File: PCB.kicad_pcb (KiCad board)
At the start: 2 copper layers, 100 x 80 mm, 31 parts, among them J1 Conn_01x04_Pin, SW1 SW_Push, SW2 SW_Push, SW3 SW_Push, SW4 SW_Push, SW5 SW_Push, SW6 SW_Push, SW7 RotaryEncoder_Switch, U1 MOUDLE-SEEEDUINO-XIAO

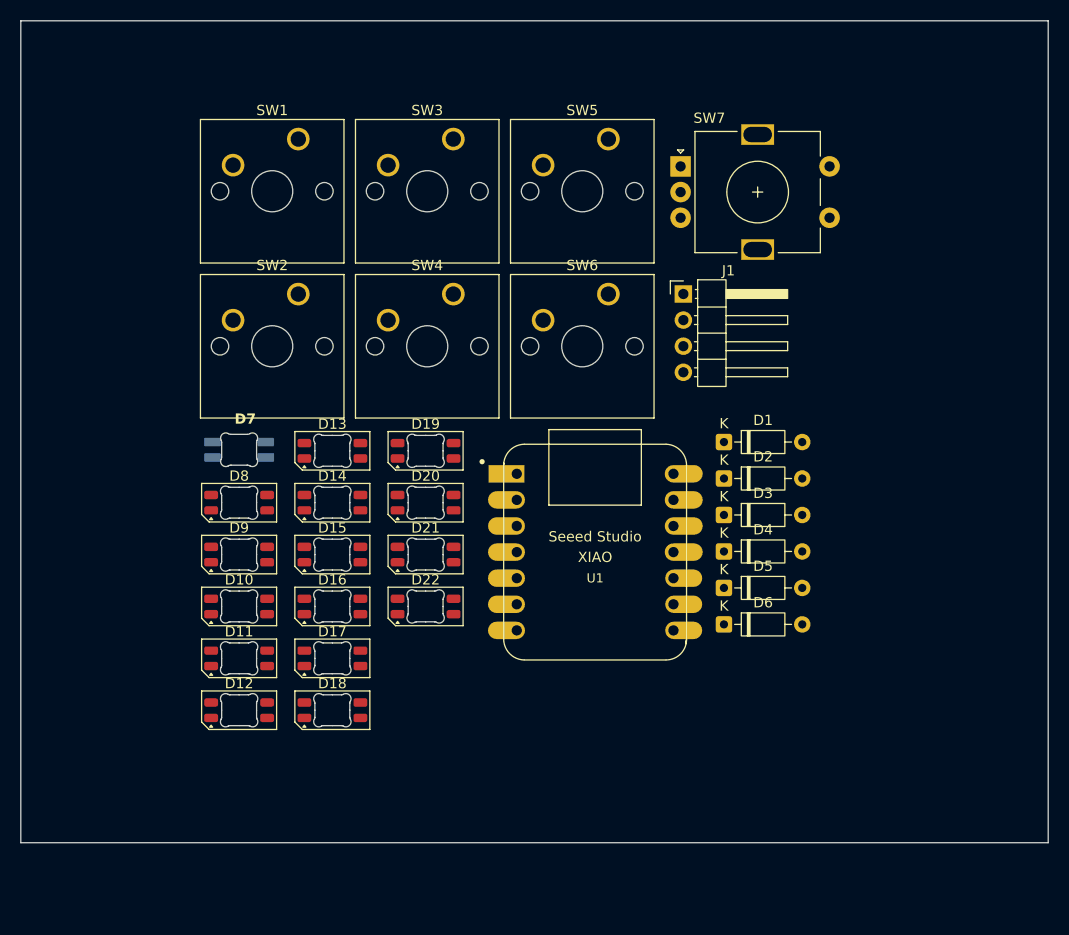
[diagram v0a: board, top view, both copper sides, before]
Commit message: PCB done
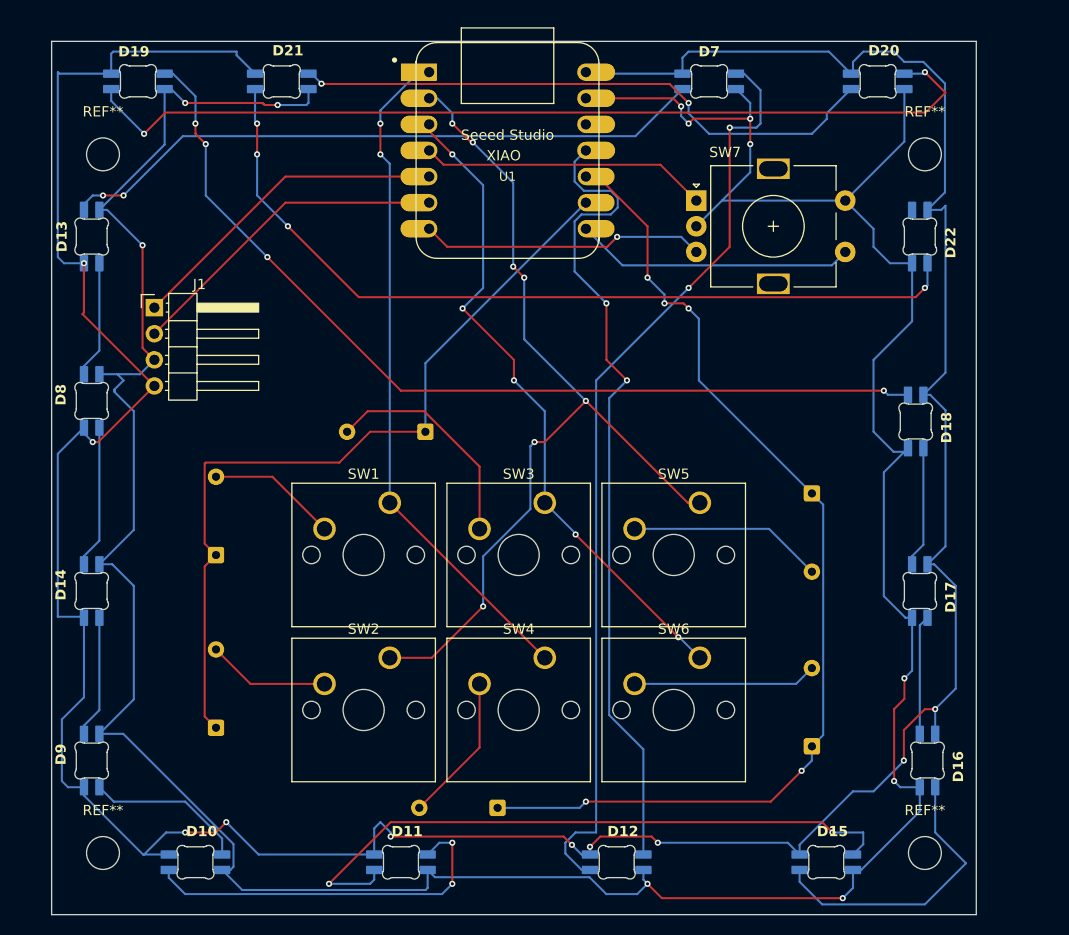
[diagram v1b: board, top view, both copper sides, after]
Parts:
- added REF**: MountingHole_3.2mm_M3, MountingHole:MountingHole_3.2mm_M3, F.Cu at (193.0, 42.0)
- added REF**: MountingHole_3.2mm_M3, MountingHole:MountingHole_3.2mm_M3, F.Cu at (113.0, 110.0)
- added REF**: MountingHole_3.2mm_M3, MountingHole:MountingHole_3.2mm_M3, F.Cu at (193.0, 110.0)
- added REF**: MountingHole_3.2mm_M3, MountingHole:MountingHole_3.2mm_M3, F.Cu at (113.0, 42.0)
- D1, D2, D3, D4, D5, D6: moved to B.Cu
- D10, D11, D12, D13, D14, D15, D16, D17, D18, D19, D20, D21, D22, D8, D9: footprint LED_SMD:LED_SK6812MINI-E_3.2x2.8mm_P1.5mm_ReverseMount -> footprints:SK6812MINI-E_fixed
- moved D18 63.3 mm to (192.0, 68.0), turned to -90 degrees
- moved D20 60.1 mm to (188.4, 35.0)
- moved D22 60.0 mm to (192.4, 50.0), turned to -90 degrees
- moved D16 59.7 mm to (193.1, 101.0), turned to -90 degrees
- moved D7 58.1 mm to (172.0, 35.0)
- moved D17 57.4 mm to (192.4, 84.5), turned to -90 degrees
- moved D15 56.7 mm to (183.4, 111.0)
- moved D2 55.1 mm to (124.0, 97.8), turned to 90 degrees
- moved J1 51.5 mm to (118.0, 56.9)
- moved D1 50.6 mm to (124.0, 81.0), turned to 90 degrees
- moved D21 48.0 mm to (130.4, 35.0)
- moved D19 45.5 mm to (116.4, 35.0)
- moved U1 40.0 mm to (152.4, 41.6)
- moved D12 39.7 mm to (163.0, 111.0)
- moved SW1 36.5 mm to (140.9, 75.9)
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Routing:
- net VCC: track 0.00 -> 327.4 mm, vias 0 -> 10
- net GND: track 0.00 -> 326.8 mm, vias 0 -> 11
- net ROW1: track 0.00 -> 101.1 mm, vias 0 -> 5
- net Net-(D12-DOUT): track 0.00 -> 91.0 mm, vias 0 -> 2
- net Net-(D18-DOUT): track 0.00 -> 90.4 mm, vias 0 -> 4
- net Net-(D19-DOUT): track 0.00 -> 90.2 mm, vias 0 -> 2
- net COL1: track 0.00 -> 87.4 mm, vias 0 -> 7
- net Net-(D21-DOUT): track 0.00 -> 82.4 mm, vias 0 -> 4
- net WS2812B: track 0.00 -> 79.9 mm, vias 0 -> 2
- net ROW0: track 0.00 -> 78.6 mm
- net COL0: track 0.00 -> 66.2 mm, vias 0 -> 2
- net COL2: track 0.00 -> 64.5 mm, vias 0 -> 5
- net Net-(D13-DIN): track 0.00 -> 63.4 mm, vias 0 -> 2
- net Net-(D11-DOUT): track 0.00 -> 63.0 mm, vias 0 -> 2
- net Net-(D20-DOUT): track 0.00 -> 58.0 mm, vias 0 -> 2
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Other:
- board size 100 x 80 mm -> 90 x 85 mm
